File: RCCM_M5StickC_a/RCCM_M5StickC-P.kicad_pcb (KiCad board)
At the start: 2 copper layers, 96.5 x 88.9 mm, 128 parts, among them CN1 Conn_02x04_Odd_Even, CN2 Conn_01x04, CN3 Conn_01x04, CN4 Conn_01x08

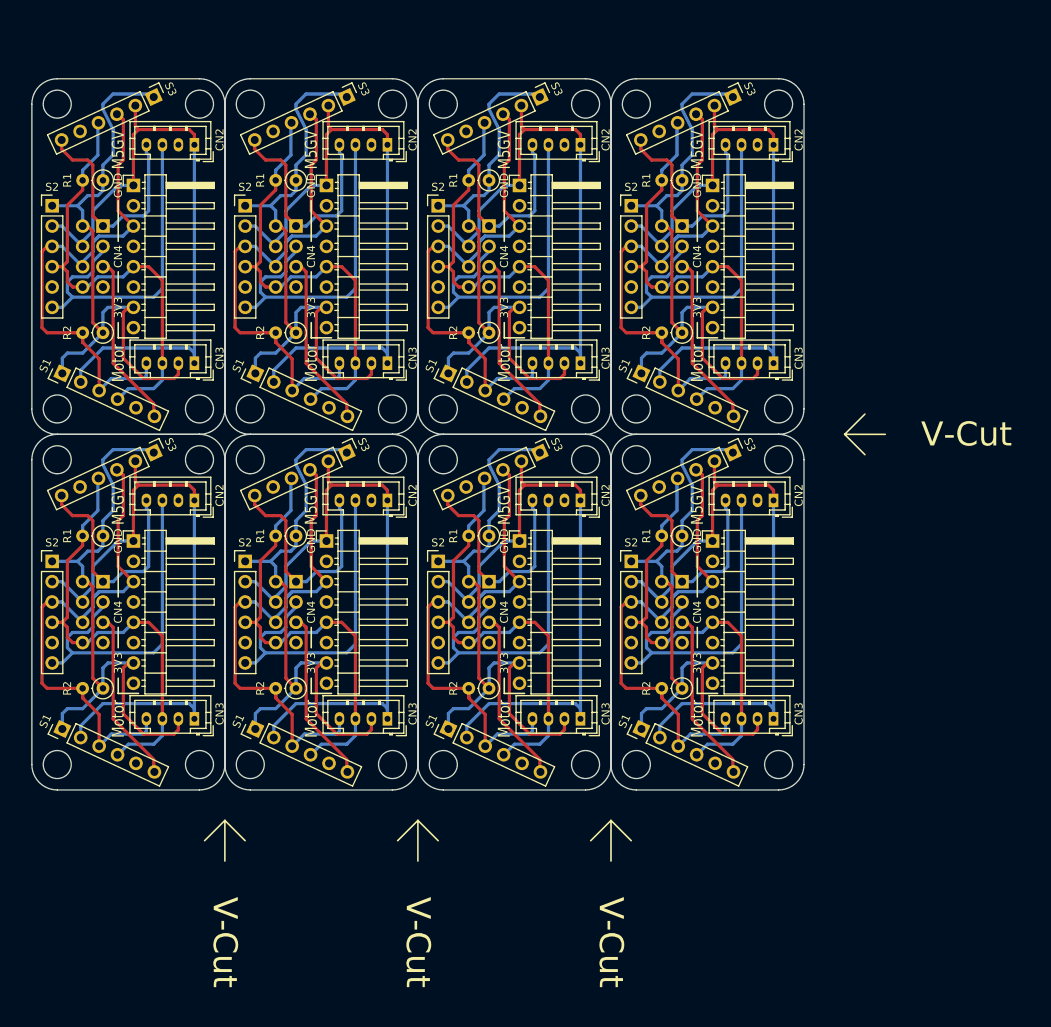
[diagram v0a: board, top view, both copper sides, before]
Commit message: Small changes
M5Stick-C Rev.a
ESP32 None
RasPi ZW  Change gerber
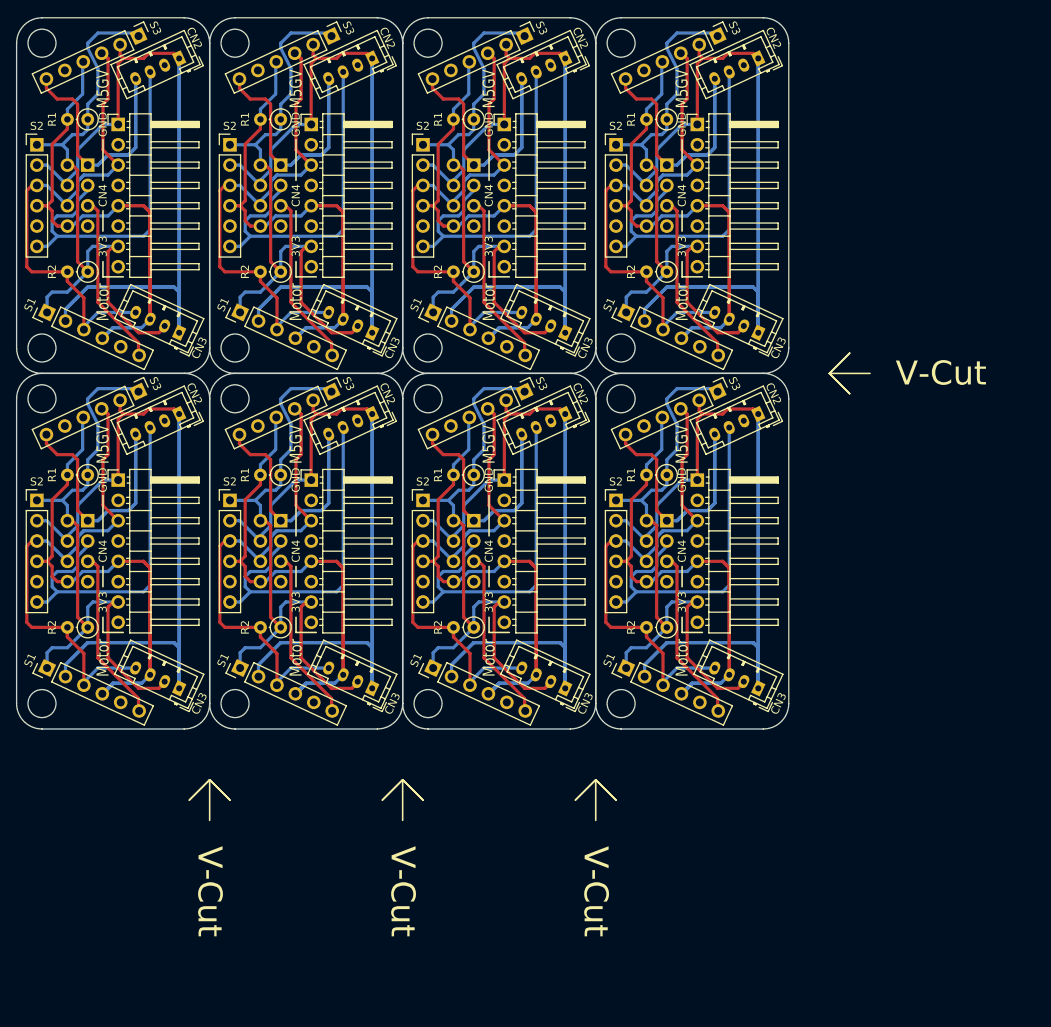
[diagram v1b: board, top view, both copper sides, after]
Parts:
- removed the CN1 at (144.8, 102.9)
- removed the CN1 at (120.7, 102.9)
- removed the CN1 at (96.5, 102.9)
- removed the CN1 at (72.4, 102.9)
- removed the CN1 at (144.8, 58.4)
- removed the CN1 at (120.7, 58.4)
- removed the CN1 at (96.5, 58.4)
- removed the CN2 at (156.2, 92.7)
- removed the CN2 at (132.1, 92.7)
- removed the CN2 at (108.0, 92.7)
- removed the CN2 at (83.8, 92.7)
- removed the CN2 at (156.2, 48.3)
- removed the CN2 at (132.1, 48.3)
- removed the CN2 at (108.0, 48.3)
- removed the CN3 at (156.2, 120.0)
- removed the CN3 at (132.1, 120.0)
- removed the CN3 at (108.0, 120.0)
- removed the CN3 at (83.8, 120.0)
- removed the CN3 at (156.2, 75.6)
- removed the CN3 at (132.1, 75.6)
- removed the CN3 at (108.0, 75.6)
- removed the CN4 at (148.6, 97.8)
- removed the CN4 at (124.5, 97.8)
- removed the CN4 at (100.3, 97.8)
- removed the CN4 at (76.2, 97.8)
- removed the CN4 at (148.6, 53.3)
- removed the CN4 at (124.5, 53.3)
- removed the CN4 at (100.3, 53.3)
- removed the G*** at (152.1, 108.3)
- removed the G*** at (107.3, 106.0)
- removed the G*** at (83.2, 106.0)
- removed the G*** at (155.6, 61.6)
- removed the G*** at (131.4, 61.6)
- removed the G*** at (107.3, 61.6)
- removed the G*** at (152.1, 100.6)
- removed the G*** at (128.0, 100.6)
- removed the G*** at (103.8, 100.6)
- removed the G*** at (79.7, 100.6)
- removed the G*** at (152.1, 56.2)
- removed the G*** at (128.0, 108.3)
- removed the G*** at (128.0, 56.2)
- removed the G*** at (103.8, 56.2)
- removed the G*** at (103.8, 108.3)
- removed the G*** at (79.7, 108.3)
- removed the G*** at (152.1, 63.8)
- removed the G*** at (128.0, 63.8)
- removed the G*** at (103.8, 63.8)
- removed the G*** at (155.6, 106.0)
- removed the G*** at (131.4, 106.0)
- removed the H1 at (139.1, 87.6)
- removed the H1 at (114.9, 87.6)
- removed the H1 at (90.8, 87.6)
- removed the H1 at (66.7, 87.6)
- removed the H1 at (139.1, 43.2)
- removed the H1 at (114.9, 43.2)
- removed the H1 at (90.8, 43.2)
- removed H2 (x8), H4 (x8): MountingHole_3.5mm, Mounting_Holes:MountingHole_3.5mm
- removed the H3 at (139.1, 125.7)
- removed the H3 at (114.9, 125.7)
- removed the H3 at (90.8, 125.7)
- removed the H3 at (66.7, 125.7)
- removed the H3 at (139.1, 81.3)
- removed the H3 at (114.9, 81.3)
- removed the H3 at (90.8, 81.3)
- removed the R1 at (144.8, 97.2)
- removed the R1 at (120.7, 97.2)
- removed the R1 at (96.5, 97.2)
- removed the R1 at (72.4, 97.2)
- removed the R1 at (144.8, 52.7)
- removed the R1 at (120.7, 52.7)
- removed the R1 at (96.5, 52.7)
- removed the R2 at (144.8, 116.2)
- removed the R2 at (120.7, 116.2)
- removed the R2 at (96.5, 116.2)
- removed the R2 at (72.4, 116.2)
- removed the R2 at (144.8, 71.8)
- removed the R2 at (120.7, 71.8)
- removed the R2 at (96.5, 71.8)
- removed the S1 at (139.7, 121.3)
- removed the S1 at (115.6, 121.3)
- removed the S1 at (91.4, 121.3)
- removed the S1 at (67.3, 121.3)
- removed the S1 at (139.7, 76.8)
- removed the S1 at (115.6, 76.8)
- removed the S1 at (91.4, 76.8)
- removed the S2 at (138.4, 100.3)
- removed the S2 at (114.3, 100.3)
- removed the S2 at (90.2, 100.3)
- removed the S2 at (66.0, 100.3)
- removed the S2 at (138.4, 55.9)
- removed the S2 at (114.3, 55.9)
- removed the S2 at (90.2, 55.9)
- removed the S3 at (151.1, 86.7)
- removed the S3 at (127.0, 86.7)
- removed the S3 at (102.9, 86.7)
- removed the S3 at (78.7, 86.7)
- removed the S3 at (151.1, 42.3)
- removed the S3 at (127.0, 42.3)
- removed the S3 at (102.9, 42.3)
- added CN1: Conn_02x04_Odd_Even, Pin_Headers:Pin_Header_Straight_2x04_Pitch2.54mm, B.Cu at (142.9, 95.2)
- added CN1: Conn_02x04_Odd_Even, Pin_Headers:Pin_Header_Straight_2x04_Pitch2.54mm, B.Cu at (118.7, 95.2)
- added CN1: Conn_02x04_Odd_Even, Pin_Headers:Pin_Header_Straight_2x04_Pitch2.54mm, B.Cu at (94.6, 95.2)
- added CN1: Conn_02x04_Odd_Even, Pin_Headers:Pin_Header_Straight_2x04_Pitch2.54mm, B.Cu at (70.5, 95.2)
- added CN1: Conn_02x04_Odd_Even, Pin_Headers:Pin_Header_Straight_2x04_Pitch2.54mm, B.Cu at (142.9, 50.8)
- added CN1: Conn_02x04_Odd_Even, Pin_Headers:Pin_Header_Straight_2x04_Pitch2.54mm, B.Cu at (118.7, 50.8)
- added CN1: Conn_02x04_Odd_Even, Pin_Headers:Pin_Header_Straight_2x04_Pitch2.54mm, B.Cu at (94.6, 50.8)
- added CN2: Conn_01x04, Connectors_JST:JST_PH_B4B-PH-K_04x2.00mm_Straight, F.Cu at (154.3, 81.9)
- added CN2: Conn_01x04, Connectors_JST:JST_PH_B4B-PH-K_04x2.00mm_Straight, F.Cu at (130.2, 81.9)
- added CN2: Conn_01x04, Connectors_JST:JST_PH_B4B-PH-K_04x2.00mm_Straight, F.Cu at (106.0, 81.9)
- added CN2: Conn_01x04, Connectors_JST:JST_PH_B4B-PH-K_04x2.00mm_Straight, F.Cu at (81.9, 81.9)
- added CN2: Conn_01x04, Connectors_JST:JST_PH_B4B-PH-K_04x2.00mm_Straight, F.Cu at (154.3, 37.5)
- added CN2: Conn_01x04, Connectors_JST:JST_PH_B4B-PH-K_04x2.00mm_Straight, F.Cu at (130.2, 37.5)
- added CN2: Conn_01x04, Connectors_JST:JST_PH_B4B-PH-K_04x2.00mm_Straight, F.Cu at (106.0, 37.5)
- added CN3: Conn_01x04, Connectors_JST:JST_PH_B4B-PH-K_04x2.00mm_Straight, F.Cu at (154.3, 116.2)
- added CN3: Conn_01x04, Connectors_JST:JST_PH_B4B-PH-K_04x2.00mm_Straight, F.Cu at (130.2, 116.2)
- added CN3: Conn_01x04, Connectors_JST:JST_PH_B4B-PH-K_04x2.00mm_Straight, F.Cu at (106.0, 116.2)
- added CN3: Conn_01x04, Connectors_JST:JST_PH_B4B-PH-K_04x2.00mm_Straight, F.Cu at (81.9, 116.2)
- added CN3: Conn_01x04, Connectors_JST:JST_PH_B4B-PH-K_04x2.00mm_Straight, F.Cu at (154.3, 71.8)
- added CN3: Conn_01x04, Connectors_JST:JST_PH_B4B-PH-K_04x2.00mm_Straight, F.Cu at (130.2, 71.8)
- added CN3: Conn_01x04, Connectors_JST:JST_PH_B4B-PH-K_04x2.00mm_Straight, F.Cu at (106.0, 71.8)
- added CN4: Conn_01x08, Pin_Headers:Pin_Header_Angled_1x08_Pitch2.54mm, F.Cu at (146.7, 90.2)
- added CN4: Conn_01x08, Pin_Headers:Pin_Header_Angled_1x08_Pitch2.54mm, F.Cu at (122.6, 90.2)
- added CN4: Conn_01x08, Pin_Headers:Pin_Header_Angled_1x08_Pitch2.54mm, F.Cu at (98.4, 90.2)
- added CN4: Conn_01x08, Pin_Headers:Pin_Header_Angled_1x08_Pitch2.54mm, F.Cu at (74.3, 90.2)
- added CN4: Conn_01x08, Pin_Headers:Pin_Header_Angled_1x08_Pitch2.54mm, F.Cu at (146.7, 45.7)
- added CN4: Conn_01x08, Pin_Headers:Pin_Header_Angled_1x08_Pitch2.54mm, F.Cu at (122.6, 45.7)
- added CN4: Conn_01x08, Pin_Headers:Pin_Header_Angled_1x08_Pitch2.54mm, F.Cu at (98.4, 45.7)
- added G***: LOGO, logos:RumiCar2_3p3, B.Cu at (150.2, 100.6)
- added G***: LOGO, logos:ALGYAN2p5, B.Cu at (105.4, 98.4)
- added G***: LOGO, logos:ALGYAN2p5, B.Cu at (81.3, 98.4)
- added G***: LOGO, logos:ALGYAN2p5, B.Cu at (153.7, 54.0)
- added G***: LOGO, logos:ALGYAN2p5, B.Cu at (129.5, 54.0)
- added G***: LOGO, logos:ALGYAN2p5, B.Cu at (105.4, 54.0)
- added G***: LOGO, logos:RumiCar1_3p3, B.Cu at (150.2, 93.0)
- added G***: LOGO, logos:RumiCar1_3p3, B.Cu at (126.0, 93.0)
- added G***: LOGO, logos:RumiCar1_3p3, B.Cu at (101.9, 93.0)
- added G***: LOGO, logos:RumiCar1_3p3, B.Cu at (77.8, 93.0)
- added G***: LOGO, logos:RumiCar1_3p3, B.Cu at (150.2, 48.6)
- added G***: LOGO, logos:RumiCar2_3p3, B.Cu at (126.0, 100.6)
- added G***: LOGO, logos:RumiCar1_3p3, B.Cu at (126.0, 48.6)
- added G***: LOGO, logos:RumiCar1_3p3, B.Cu at (101.9, 48.6)
- added G***: LOGO, logos:RumiCar2_3p3, B.Cu at (101.9, 100.6)
- added G***: LOGO, logos:RumiCar2_3p3, B.Cu at (77.8, 100.6)
- added G***: LOGO, logos:RumiCar2_3p3, B.Cu at (150.2, 56.2)
- added G***: LOGO, logos:RumiCar2_3p3, B.Cu at (126.0, 56.2)
- added G***: LOGO, logos:RumiCar2_3p3, B.Cu at (101.9, 56.2)
- added G***: LOGO, logos:ALGYAN2p5, B.Cu at (153.7, 98.4)
- added G***: LOGO, logos:ALGYAN2p5, B.Cu at (129.5, 98.4)
- added H1: MountingHole_3.5mm, Mounting_Holes:MountingHole_3.5mm, F.Cu at (137.2, 80.0)
- added H1: MountingHole_3.5mm, Mounting_Holes:MountingHole_3.5mm, F.Cu at (113.0, 80.0)
- added H1: MountingHole_3.5mm, Mounting_Holes:MountingHole_3.5mm, F.Cu at (88.9, 80.0)
- added H1: MountingHole_3.5mm, Mounting_Holes:MountingHole_3.5mm, F.Cu at (64.8, 80.0)
- added H1: MountingHole_3.5mm, Mounting_Holes:MountingHole_3.5mm, F.Cu at (137.2, 35.6)
- added H1: MountingHole_3.5mm, Mounting_Holes:MountingHole_3.5mm, F.Cu at (113.0, 35.6)
- added H1: MountingHole_3.5mm, Mounting_Holes:MountingHole_3.5mm, F.Cu at (88.9, 35.6)
- added H3: MountingHole_3.5mm, Mounting_Holes:MountingHole_3.5mm, F.Cu at (137.2, 118.1)
- added H3: MountingHole_3.5mm, Mounting_Holes:MountingHole_3.5mm, F.Cu at (113.0, 118.1)
- added H3: MountingHole_3.5mm, Mounting_Holes:MountingHole_3.5mm, F.Cu at (88.9, 118.1)
- added H3: MountingHole_3.5mm, Mounting_Holes:MountingHole_3.5mm, F.Cu at (64.8, 118.1)
- added H3: MountingHole_3.5mm, Mounting_Holes:MountingHole_3.5mm, F.Cu at (137.2, 73.7)
- added H3: MountingHole_3.5mm, Mounting_Holes:MountingHole_3.5mm, F.Cu at (113.0, 73.7)
- added H3: MountingHole_3.5mm, Mounting_Holes:MountingHole_3.5mm, F.Cu at (88.9, 73.7)
- added R1: R, Resistors_THT:R_Axial_DIN0207_L6.3mm_D2.5mm_P2.54mm_Vertical, F.Cu at (142.9, 89.5)
- added R1: R, Resistors_THT:R_Axial_DIN0207_L6.3mm_D2.5mm_P2.54mm_Vertical, F.Cu at (118.7, 89.5)
- added R1: R, Resistors_THT:R_Axial_DIN0207_L6.3mm_D2.5mm_P2.54mm_Vertical, F.Cu at (94.6, 89.5)
- added R1: R, Resistors_THT:R_Axial_DIN0207_L6.3mm_D2.5mm_P2.54mm_Vertical, F.Cu at (70.5, 89.5)
- added R1: R, Resistors_THT:R_Axial_DIN0207_L6.3mm_D2.5mm_P2.54mm_Vertical, F.Cu at (142.9, 45.1)
- added R1: R, Resistors_THT:R_Axial_DIN0207_L6.3mm_D2.5mm_P2.54mm_Vertical, F.Cu at (118.7, 45.1)
- added R1: R, Resistors_THT:R_Axial_DIN0207_L6.3mm_D2.5mm_P2.54mm_Vertical, F.Cu at (94.6, 45.1)
- added R2: R, Resistors_THT:R_Axial_DIN0207_L6.3mm_D2.5mm_P2.54mm_Vertical, F.Cu at (142.9, 108.6)
- added R2: R, Resistors_THT:R_Axial_DIN0207_L6.3mm_D2.5mm_P2.54mm_Vertical, F.Cu at (118.7, 108.6)
- added R2: R, Resistors_THT:R_Axial_DIN0207_L6.3mm_D2.5mm_P2.54mm_Vertical, F.Cu at (94.6, 108.6)
- added R2: R, Resistors_THT:R_Axial_DIN0207_L6.3mm_D2.5mm_P2.54mm_Vertical, F.Cu at (70.5, 108.6)
- added R2: R, Resistors_THT:R_Axial_DIN0207_L6.3mm_D2.5mm_P2.54mm_Vertical, F.Cu at (142.9, 64.1)
- added R2: R, Resistors_THT:R_Axial_DIN0207_L6.3mm_D2.5mm_P2.54mm_Vertical, F.Cu at (118.7, 64.1)
- added R2: R, Resistors_THT:R_Axial_DIN0207_L6.3mm_D2.5mm_P2.54mm_Vertical, F.Cu at (94.6, 64.1)
- added S1: Conn_01x06, Pin_Headers:Pin_Header_Straight_1x06_Pitch2.54mm, F.Cu at (137.8, 113.7)
- added S1: Conn_01x06, Pin_Headers:Pin_Header_Straight_1x06_Pitch2.54mm, F.Cu at (113.7, 113.7)
- added S1: Conn_01x06, Pin_Headers:Pin_Header_Straight_1x06_Pitch2.54mm, F.Cu at (89.5, 113.7)
- added S1: Conn_01x06, Pin_Headers:Pin_Header_Straight_1x06_Pitch2.54mm, F.Cu at (65.4, 113.7)
- added S1: Conn_01x06, Pin_Headers:Pin_Header_Straight_1x06_Pitch2.54mm, F.Cu at (137.8, 69.2)
- added S1: Conn_01x06, Pin_Headers:Pin_Header_Straight_1x06_Pitch2.54mm, F.Cu at (113.7, 69.2)
- added S1: Conn_01x06, Pin_Headers:Pin_Header_Straight_1x06_Pitch2.54mm, F.Cu at (89.5, 69.2)
- added S2: Conn_01x06, Pin_Headers:Pin_Header_Straight_1x06_Pitch2.54mm, F.Cu at (136.5, 92.7)
- added S2: Conn_01x06, Pin_Headers:Pin_Header_Straight_1x06_Pitch2.54mm, F.Cu at (112.4, 92.7)
- added S2: Conn_01x06, Pin_Headers:Pin_Header_Straight_1x06_Pitch2.54mm, F.Cu at (88.3, 92.7)
- added S2: Conn_01x06, Pin_Headers:Pin_Header_Straight_1x06_Pitch2.54mm, F.Cu at (64.1, 92.7)
- added S2: Conn_01x06, Pin_Headers:Pin_Header_Straight_1x06_Pitch2.54mm, F.Cu at (136.5, 48.3)
- added S2: Conn_01x06, Pin_Headers:Pin_Header_Straight_1x06_Pitch2.54mm, F.Cu at (112.4, 48.3)
- added S2: Conn_01x06, Pin_Headers:Pin_Header_Straight_1x06_Pitch2.54mm, F.Cu at (88.3, 48.3)
- added S3: Conn_01x06, Pin_Headers:Pin_Header_Straight_1x06_Pitch2.54mm, F.Cu at (149.2, 79.1)
- added S3: Conn_01x06, Pin_Headers:Pin_Header_Straight_1x06_Pitch2.54mm, F.Cu at (125.1, 79.1)
- added S3: Conn_01x06, Pin_Headers:Pin_Header_Straight_1x06_Pitch2.54mm, F.Cu at (101.0, 79.1)
- added S3: Conn_01x06, Pin_Headers:Pin_Header_Straight_1x06_Pitch2.54mm, F.Cu at (76.8, 79.1)
- added S3: Conn_01x06, Pin_Headers:Pin_Header_Straight_1x06_Pitch2.54mm, F.Cu at (149.2, 34.7)
- added S3: Conn_01x06, Pin_Headers:Pin_Header_Straight_1x06_Pitch2.54mm, F.Cu at (125.1, 34.7)
- added S3: Conn_01x06, Pin_Headers:Pin_Header_Straight_1x06_Pitch2.54mm, F.Cu at (101.0, 34.7)
- moved CN2 11.0 mm to (81.9, 37.5), turned to 205 degrees
- moved CN1 7.85 mm to (70.5, 50.8)
- moved CN4 7.85 mm to (74.3, 45.7)
- moved G*** 7.85 mm to (77.8, 56.2)
- moved H3 7.85 mm to (64.8, 73.7)
- moved S2 7.85 mm to (64.1, 48.3)
- moved G*** 7.85 mm to (81.3, 54.0)
- moved G*** 7.85 mm to (77.8, 48.6)
- moved H1 7.85 mm to (64.8, 35.6)
- moved R1 7.85 mm to (70.5, 45.1)
- moved S3 7.85 mm to (76.8, 34.7)
- moved R2 7.85 mm to (70.5, 64.1)
- moved S1 7.85 mm to (65.4, 69.2)
- moved CN3 4.26 mm to (81.9, 71.8), turned to 155 degrees
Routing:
- net GND: track 646.5 -> 1113.0 mm
- net G00: track 450.0 -> 647.7 mm
- net G33: track 231.1 -> 345.1 mm
- net G32: track 338.3 -> 349.4 mm
- net G26: track 517.2 -> 512.0 mm
- net 3V3m: track 608.0 -> 609.4 mm
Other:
- outline, holes or cut-outs redrawn
